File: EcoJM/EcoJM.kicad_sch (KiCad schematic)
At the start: 0 parts

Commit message: bahr updoad
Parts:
- added C1: 1n, symbol Device:C
- added C2, C4, C5: 100n, symbol Device:C
- added C3: 4.7n, symbol Device:C
- added R1: 10k, symbol Device:R
- added U1, U2: ACS712xLCTR-30A, Package_SO:SOIC-8_3.9x4.9mm_P1.27mm, symbol Sensor_Current:ACS712xLCTR-30A
- added U3: SIT65HVD230DR, EasyEDA:SOP-8_L4.9-W3.9-P1.27-LS6.0-BL, symbol EasyEDA:SIT65HVD230DR
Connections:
- new net: R1.1, U3.8 (RS)
- new net: C1.1, U1.6 (FILTER)
- new net: C3.1, U2.6 (FILTER)
- new net: U2.1 (IP+), U2.2 (IP+)
- new net: U2.3 (IP-), U2.4 (IP-)
- new net: U1.1 (IP+), U1.2 (IP+)
- new net: U1.3 (IP-), U1.4 (IP-)
- new net +3.3V: C5.2, U3.3 (VCC)
- new net +5V: C2.2, C4.2, U1.8 (VCC), U2.8 (VCC)
- new net GND: C1.2, C2.1, C3.2, C4.1, C5.1, R1.2, U1.5 (GND), U2.5 (GND), U3.2 (GND)

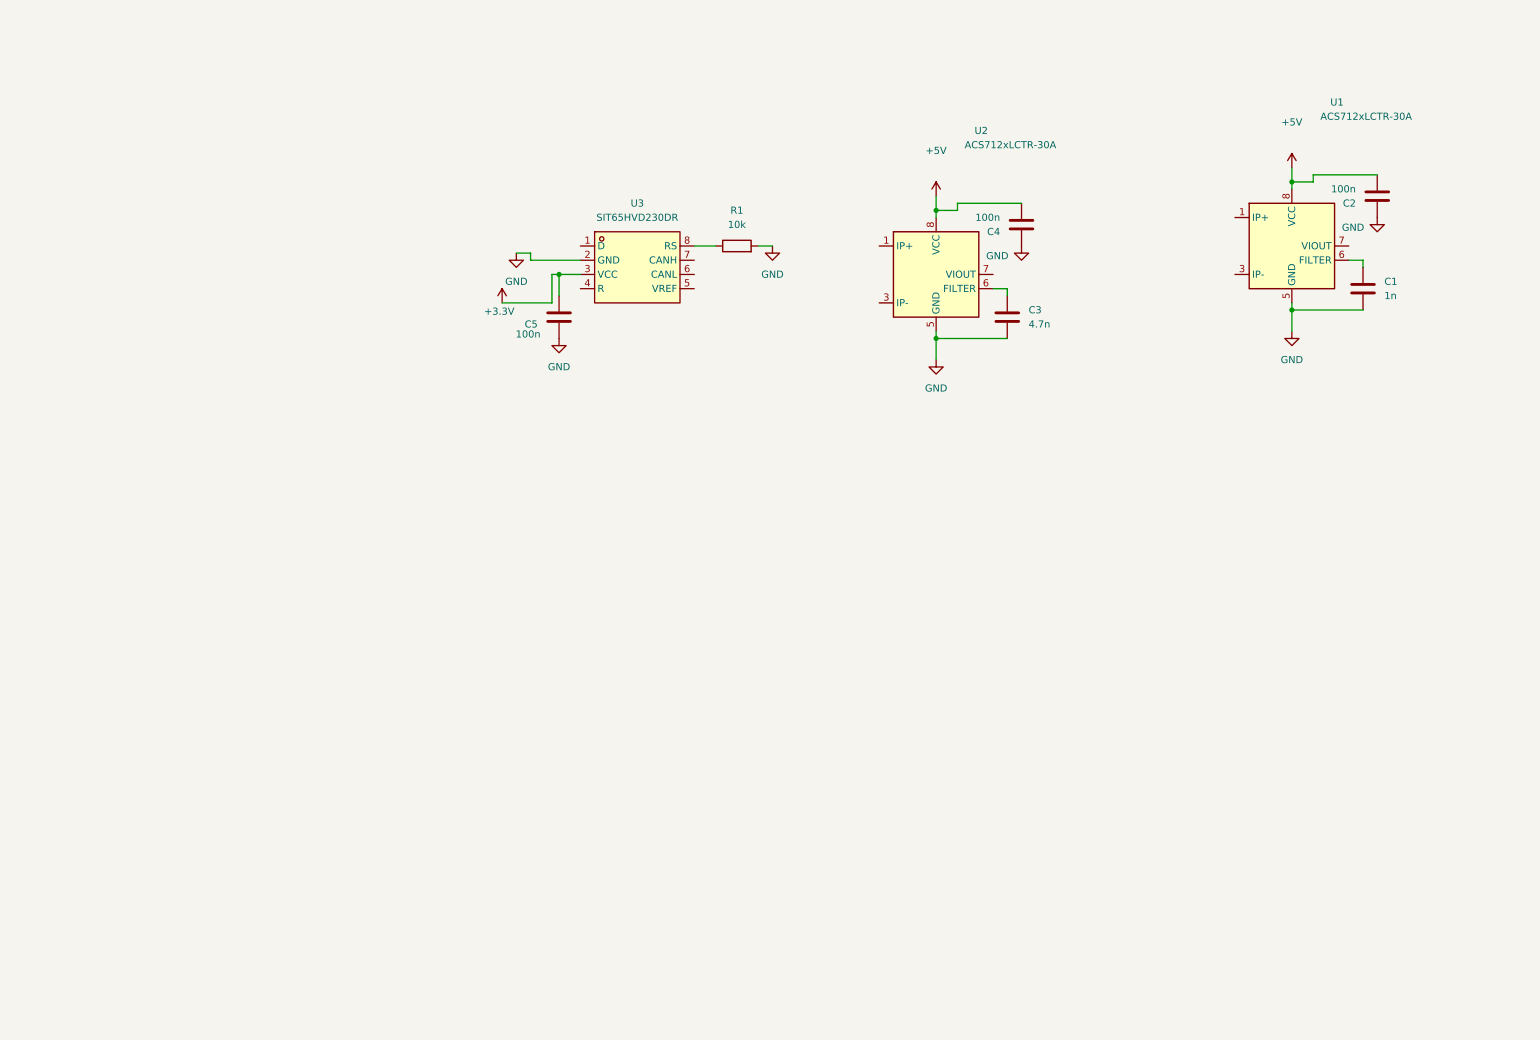
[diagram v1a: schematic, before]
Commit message: Signed-off-by: Omar-Magdy0 <omar.magdy.om.om@gmail.com> Major Updates
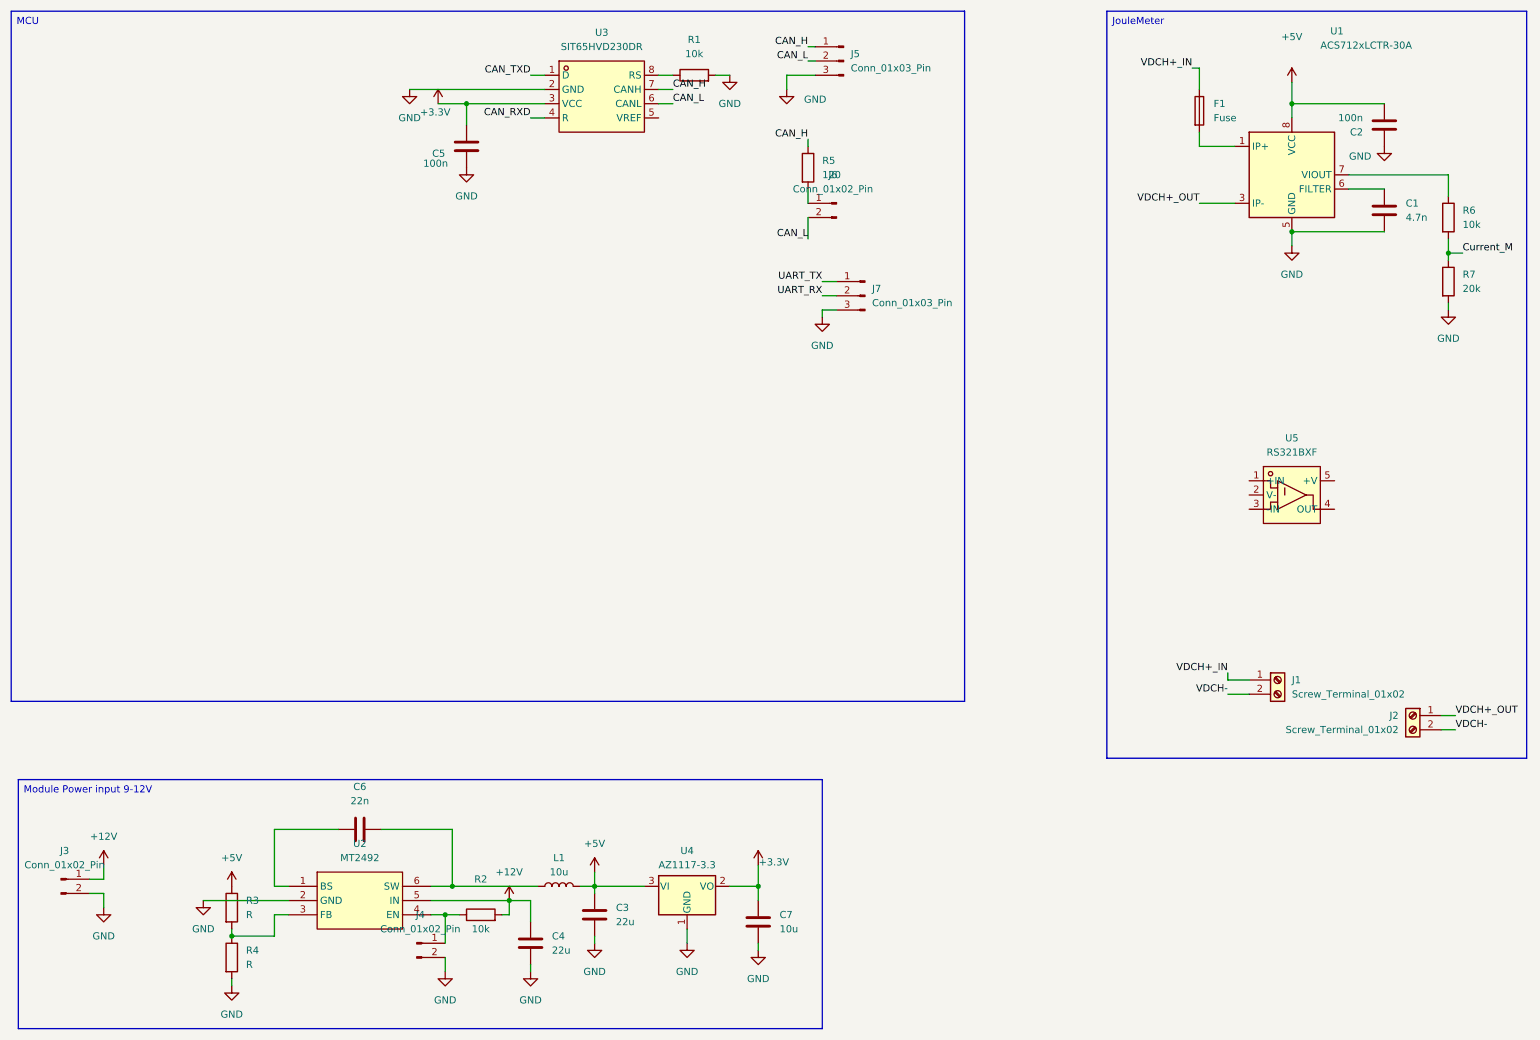
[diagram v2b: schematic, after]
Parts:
- removed U2: ACS712xLCTR-30A, Package_SO:SOIC-8_3.9x4.9mm_P1.27mm, symbol Sensor_Current:ACS712xLCTR-30A
- added C6: 22n, symbol Device:C
- added C7: 10u, symbol Device:C
- added F1: Fuse, Fuse:Fuseholder_Clip-5x20mm_Keystone_3512_Inline_P23.62x7.27mm_D1.02x1.57mm_Horizontal, symbol Device:Fuse
- added J1, J2: Screw_Terminal_01x02, symbol Connector:Screw_Terminal_01x02
- added J3, J4, J6: Conn_01x02_Pin, symbol Connector:Conn_01x02_Pin
- added J5, J7: Conn_01x03_Pin, symbol Connector:Conn_01x03_Pin
- added L1: 10u, symbol Device:L
- added R2, R6: 10k, symbol Device:R
- added R3, R4: R, symbol Device:R
- added R5: 120, symbol Device:R
- added R7: 20k, symbol Device:R
- added U2: MT2492, EasyEDA:SOT-23-6_L2.9-W1.6-P0.95-LS2.8-BL_3, symbol EasyEDA:MT2492
- added U4: AZ1117-3.3, Package_TO_SOT_SMD:SOT-89-3_Handsoldering, symbol Regulator_Linear:AZ1117-3.3
- added U5: RS321BXF, EasyEDA:SOT-23-5_L2.9-W1.6-P0.95-LS2.8-BL, symbol EasyEDA:RS321BXF
- C1: value 1n -> 4.7n
- C3: value 4.7n -> 22u
- C4: value 100n -> 22u
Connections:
- net +3.3V: now also C7.1, U4.2 (VO)
- net +5V: now also C3.2, L1.2, R3.1, U4.3 (VI); no longer C4.2
- net GND: now also C3.1, C4.2, C7.2, J3.2 (Pin_2), J4.2 (Pin_2), J5.3 (Pin_3), J7.3 (Pin_3), R4.2, R7.2, U2.2 (GND), U4.1 (GND); no longer C3.2, C4.1
- net CAN_TXD: now reaches U3.1 (D)
- net CAN_RXD: now reaches U3.4 (R)
- net CAN_L: now reaches U3.6 (CANL)
- net CAN_L: now also J5.2 (Pin_2), J6.2 (Pin_2)
- net CAN_H: now reaches U3.7 (CANH)
- net CAN_H: now also J5.1 (Pin_1), R5.1
- net at U1.1 (IP+), U1.2 (IP+): now also F1.2
- net VDCH+_OUT: now reaches U1.3 (IP-), U1.4 (IP-)
- net VDCH+_OUT: now also J2.1 (Pin_1)
- net at U1.7 (VIOUT): now also R6.1
- new net: C6.2, L1.1, U2.6 (SW)
- new net: J6.1 (Pin_1), R5.2
- new net: J4.1 (Pin_1), R2.1, U2.4 (EN)
- new net: R3.2, R4.1, U2.3 (FB)
- new net: C6.1, U2.1 (BS)
- new net +12V: C4.1, J3.1 (Pin_1), R2.2, U2.5 (IN)
- new net Current_M: R6.2, R7.1
- new net UART_RX: J7.2 (Pin_2)
- new net UART_TX: J7.1 (Pin_1)
- new net VDCH+_IN: F1.1, J1.1 (Pin_1)
- new net VDCH-: J1.2 (Pin_2), J2.2 (Pin_2)
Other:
- moved on the sheet: C1, C2, C5, R1, U1, U3
